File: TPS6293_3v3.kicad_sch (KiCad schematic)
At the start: 15 parts, among them U11 TPS62933

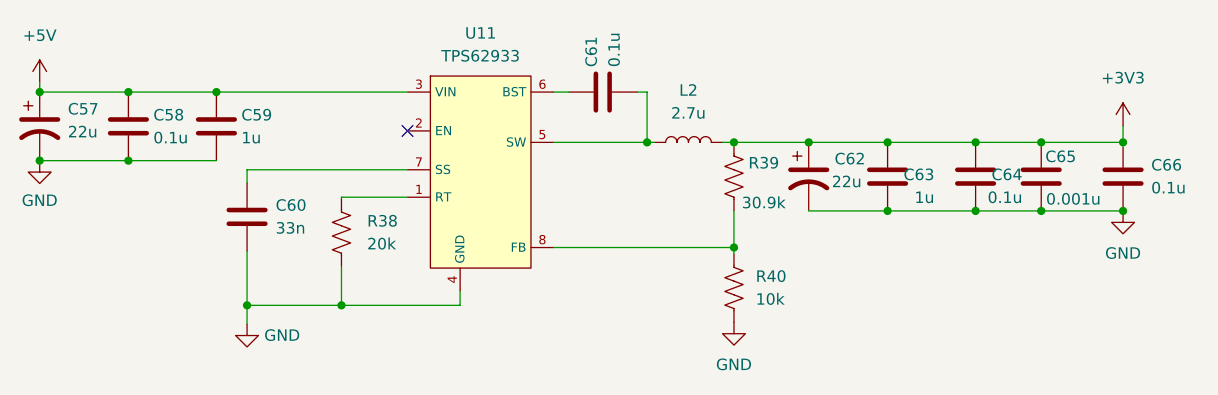
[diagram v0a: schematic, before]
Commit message: Pushing what i have now
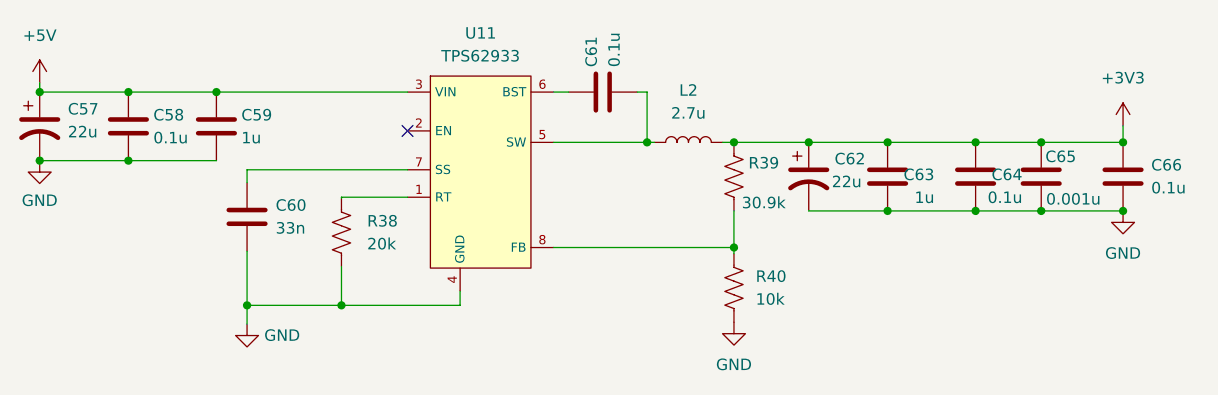
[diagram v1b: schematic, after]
